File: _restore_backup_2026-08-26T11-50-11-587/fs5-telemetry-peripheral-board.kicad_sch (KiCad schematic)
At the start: 9 parts, among them J1 ATS668LSM, U2 LM2907M/NOPB

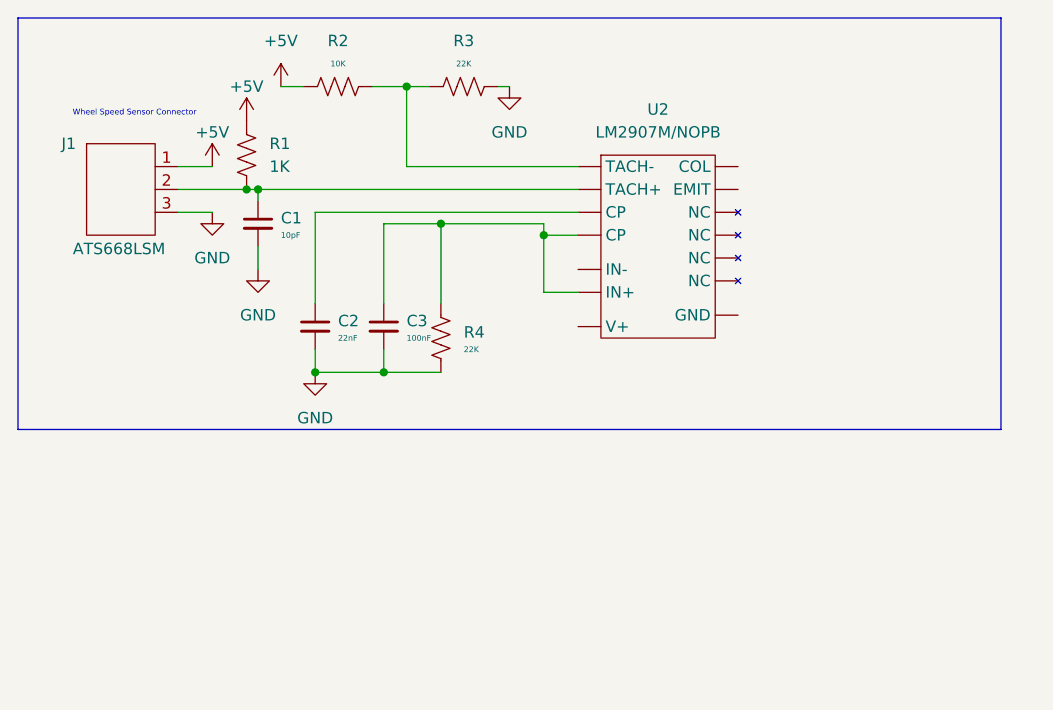
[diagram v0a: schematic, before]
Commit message: made new symbols for LM2907 and ATS668LSM
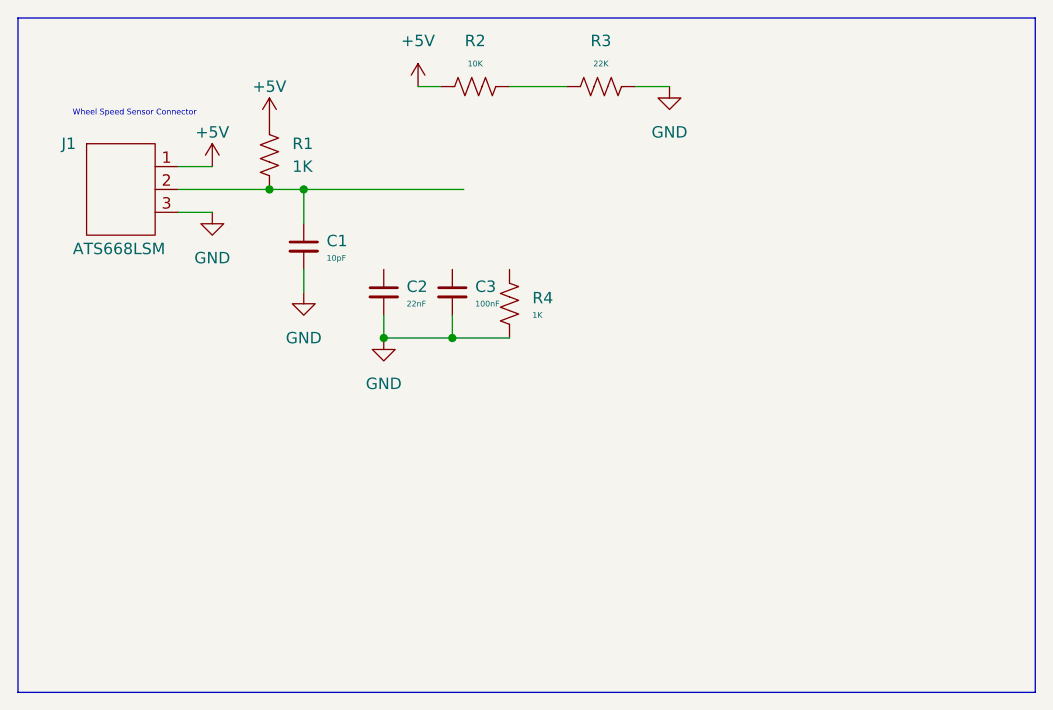
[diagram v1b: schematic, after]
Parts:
- removed U2: LM2907M/NOPB, symbol Symbols:LM2907M_NOPB
- R4: value 22K -> 1K
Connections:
- net at C3.1: no longer R4.1
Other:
- moved on the sheet: C1, C2, C3, R1, R2, R3, R4
